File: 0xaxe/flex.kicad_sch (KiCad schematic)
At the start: 39 parts, among them U4 INA500DCK, U5 INA500DCK, U6 INA500DCK, U7 INA500DCK, U8 ISL21080CIH315Z-TK, U9 LM339

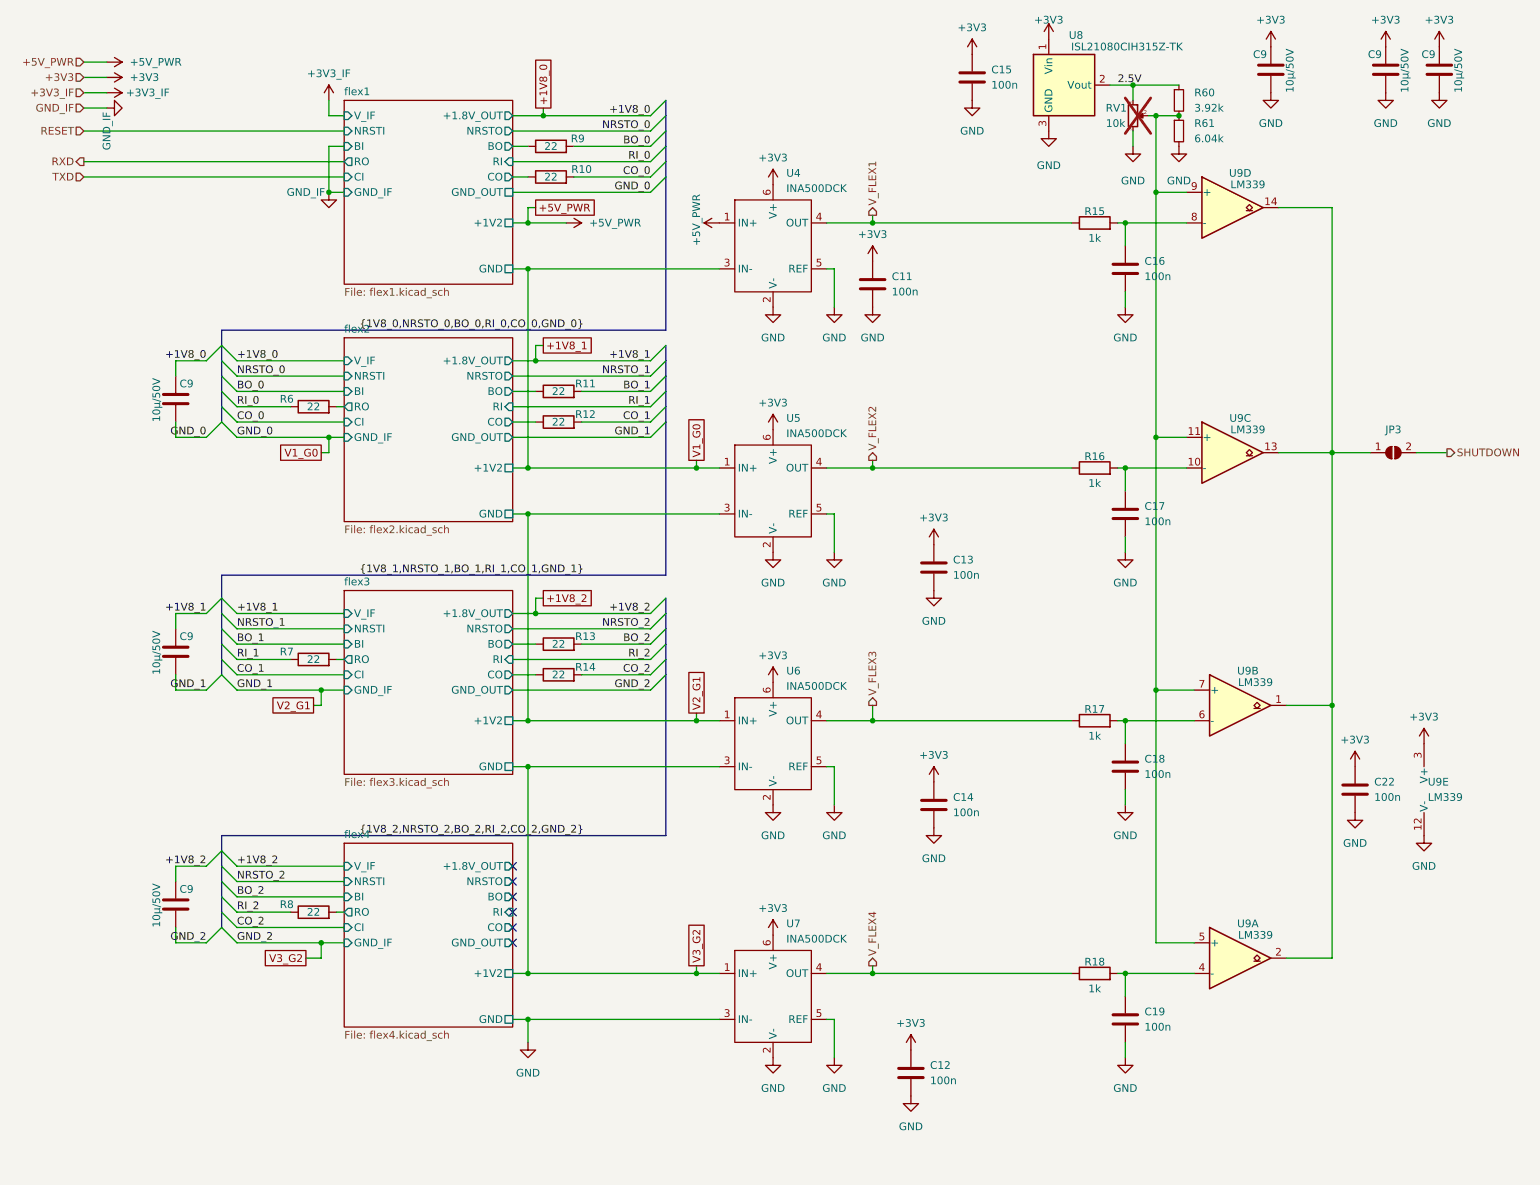
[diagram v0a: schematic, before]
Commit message: op levelshifter
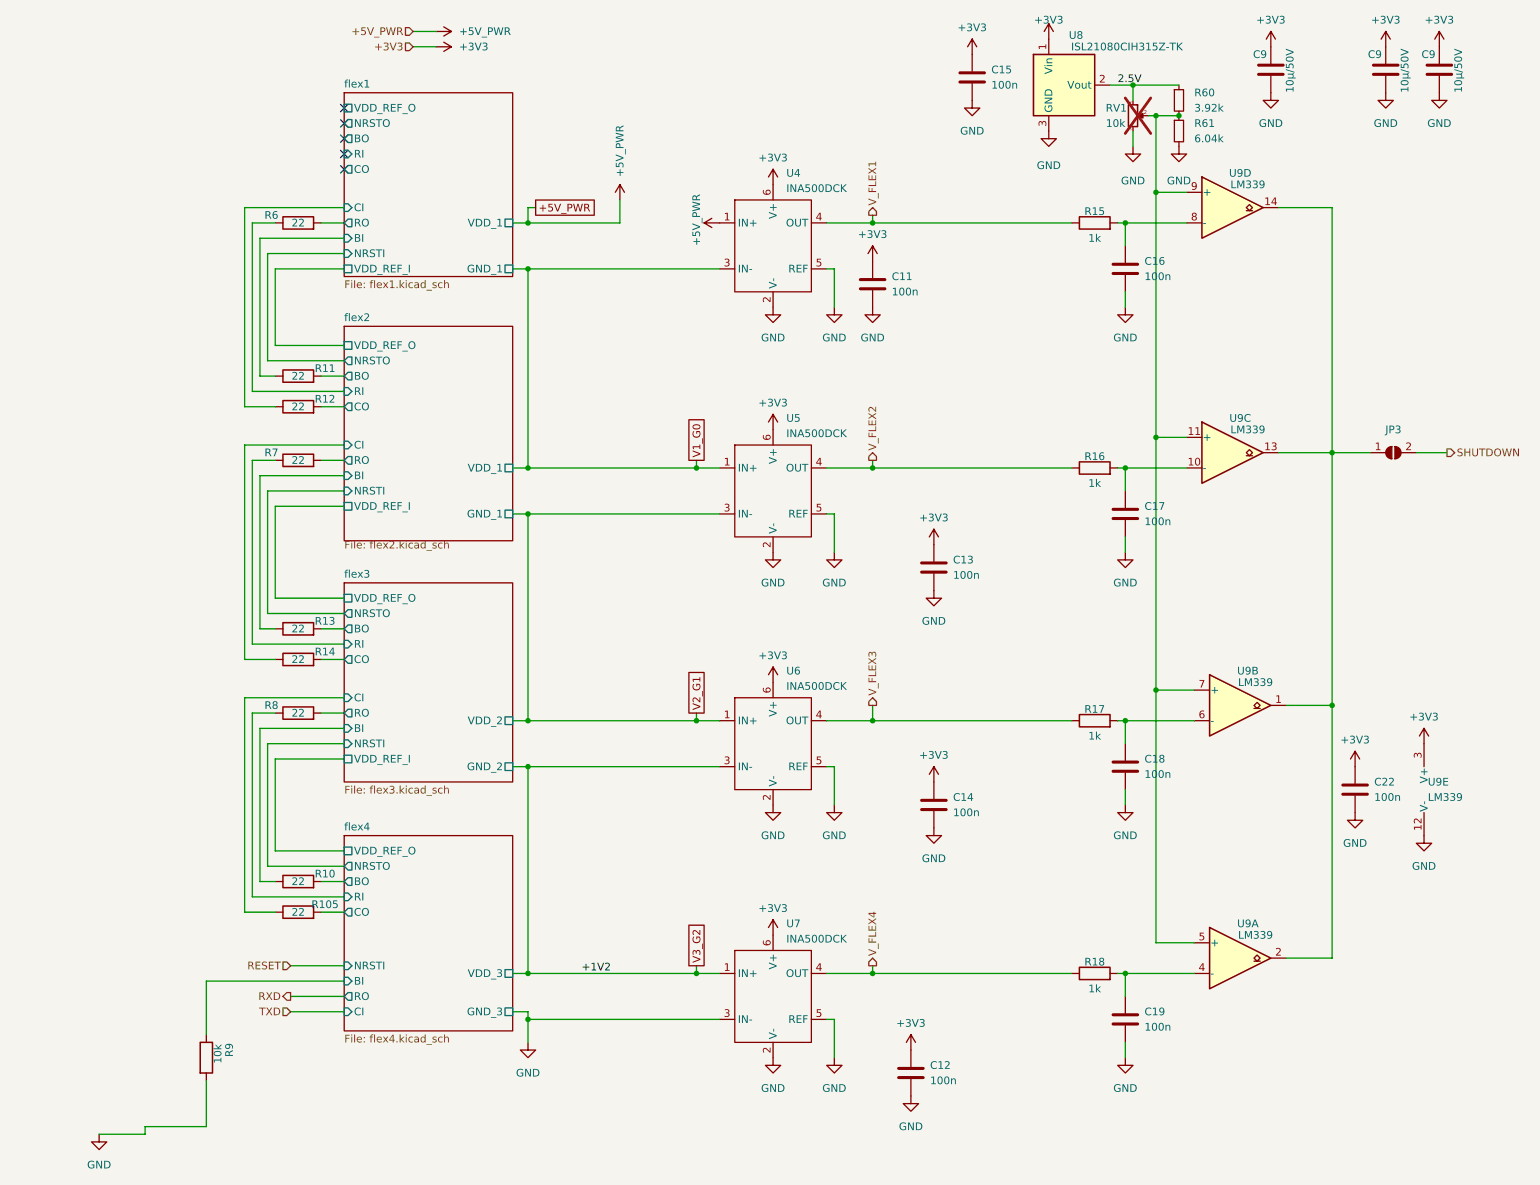
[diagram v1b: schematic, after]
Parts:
- removed C9 (x3): 10µ/50V, Capacitor_SMD:C_1206_3216Metric, symbol Device:C
- added R105: 22, Resistor_SMD:R_0805_2012Metric, symbol Device:R
- R9: value 22 -> 10k
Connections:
- net BO_0 is gone; now on net GND: R9.2
- net BO_1 is gone; now on net flex2/BO: R11.2
- net BO_2 is gone; now on net flex3/BO: R13.2
- net CO_0 is gone; now on net flex4/BO: R10.2
- net CO_1 is gone; now on net flex2/CO: R12.2
- net CO_2 is gone; now on net flex3/CO: R14.2
- net RI_2 is gone; now on net flex4/RI: R8.1
- net flex4/RO is gone; now on net flex3/RO: R8.2
- net flex1/BO: no longer R9.1
- net flex1/CO: no longer R10.1
- net flex2/BO: no longer R11.1
- net flex2/CO: no longer R12.1
- net flex2/RO: now also R7.2; no longer R6.2
- net flex3/BO: no longer R13.1
- net flex3/CO: no longer R14.1
- net flex3/RO: no longer R7.2
- net flex4/CO: now also R105.2
- net RI_0 renamed flex2/RI
- net RI_1 renamed flex3/RI
- new net flex1/BI: R11.1
- new net flex1/CI: R12.1
- new net flex1/RO: R6.2
- new net flex2/BI: R13.1
- new net flex2/CI: R14.1
- new net flex3/BI: R10.1
- new net flex3/CI: R105.1
- new net flex4/BI: R9.1
- no-connect marks 6 -> 5
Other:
- sheet flex1 ports: added GND_1, VDD_1, VDD_REF_I, VDD_REF_O; removed +1.8V_OUT, +1V2, GND, GND_IF, GND_OUT, V_IF
- sheet flex2 ports: added GND_1, VDD_1, VDD_REF_I, VDD_REF_O; removed +1.8V_OUT, +1V2, GND, GND_IF, GND_OUT, V_IF
- sheet flex3 ports: added GND_2, VDD_2, VDD_REF_I, VDD_REF_O; removed +1.8V_OUT, +1V2, GND, GND_IF, GND_OUT, V_IF
- sheet flex4 ports: added GND_3, VDD_3, VDD_REF_O; removed +1.8V_OUT, +1V2, GND, GND_IF, GND_OUT, V_IF
- moved on the sheet: R11, R12, R13, R14, R6, R7, R8
